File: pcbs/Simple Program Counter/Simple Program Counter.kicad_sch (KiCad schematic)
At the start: 0 parts

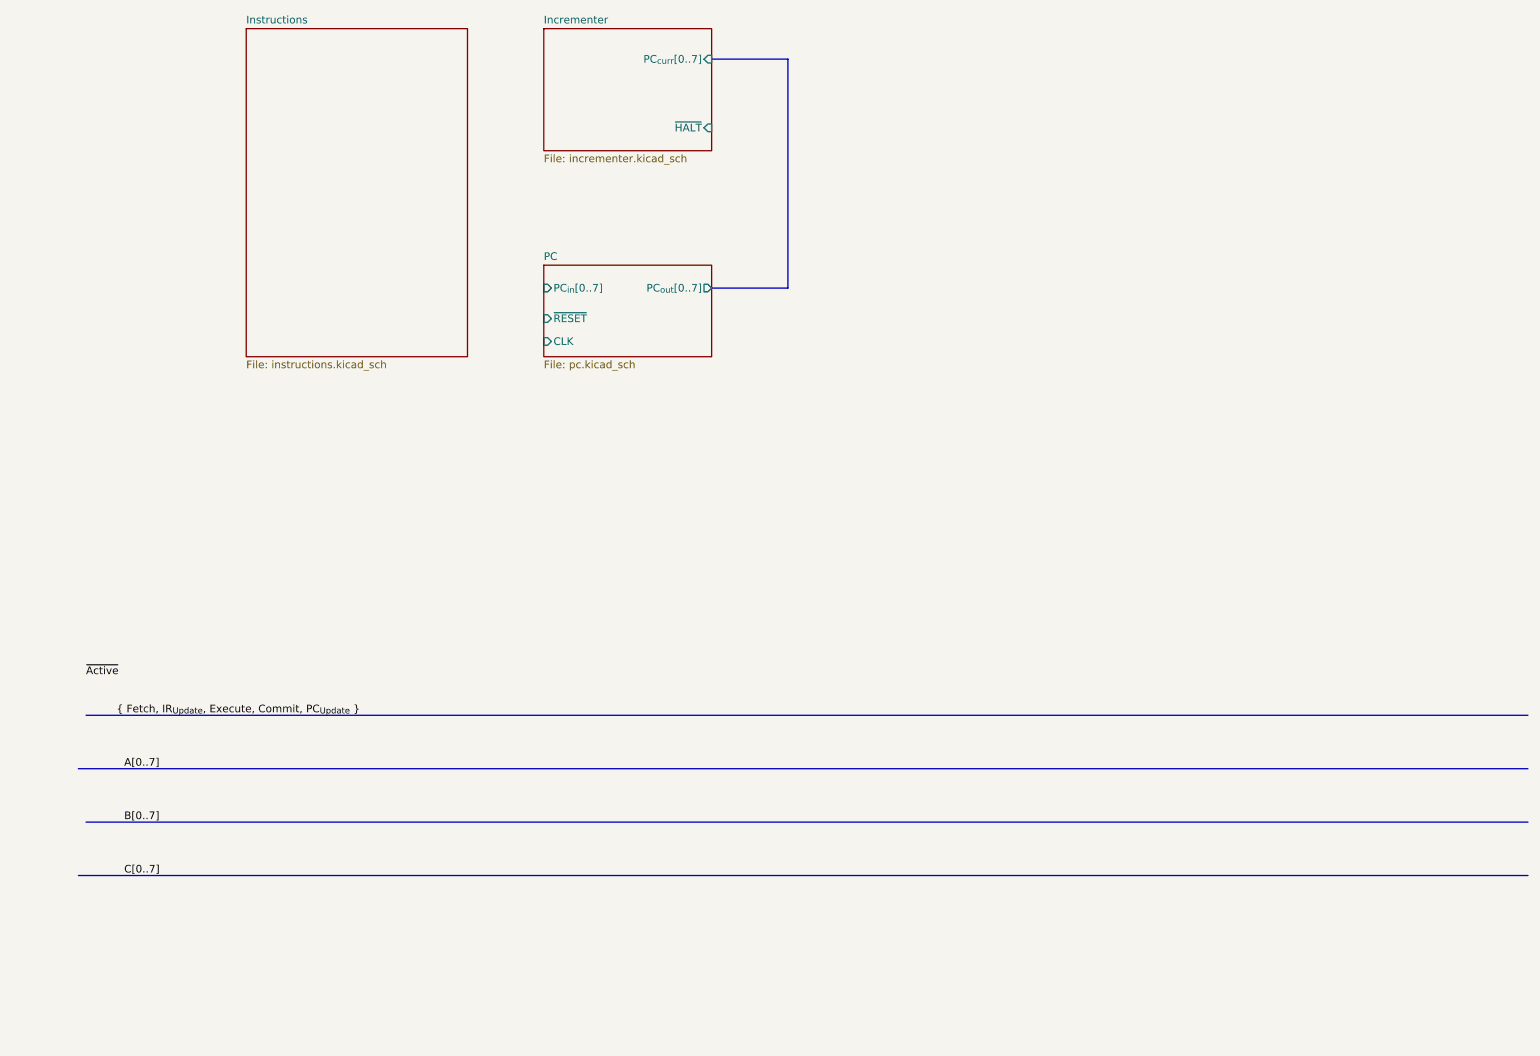
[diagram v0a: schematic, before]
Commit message: Getting close
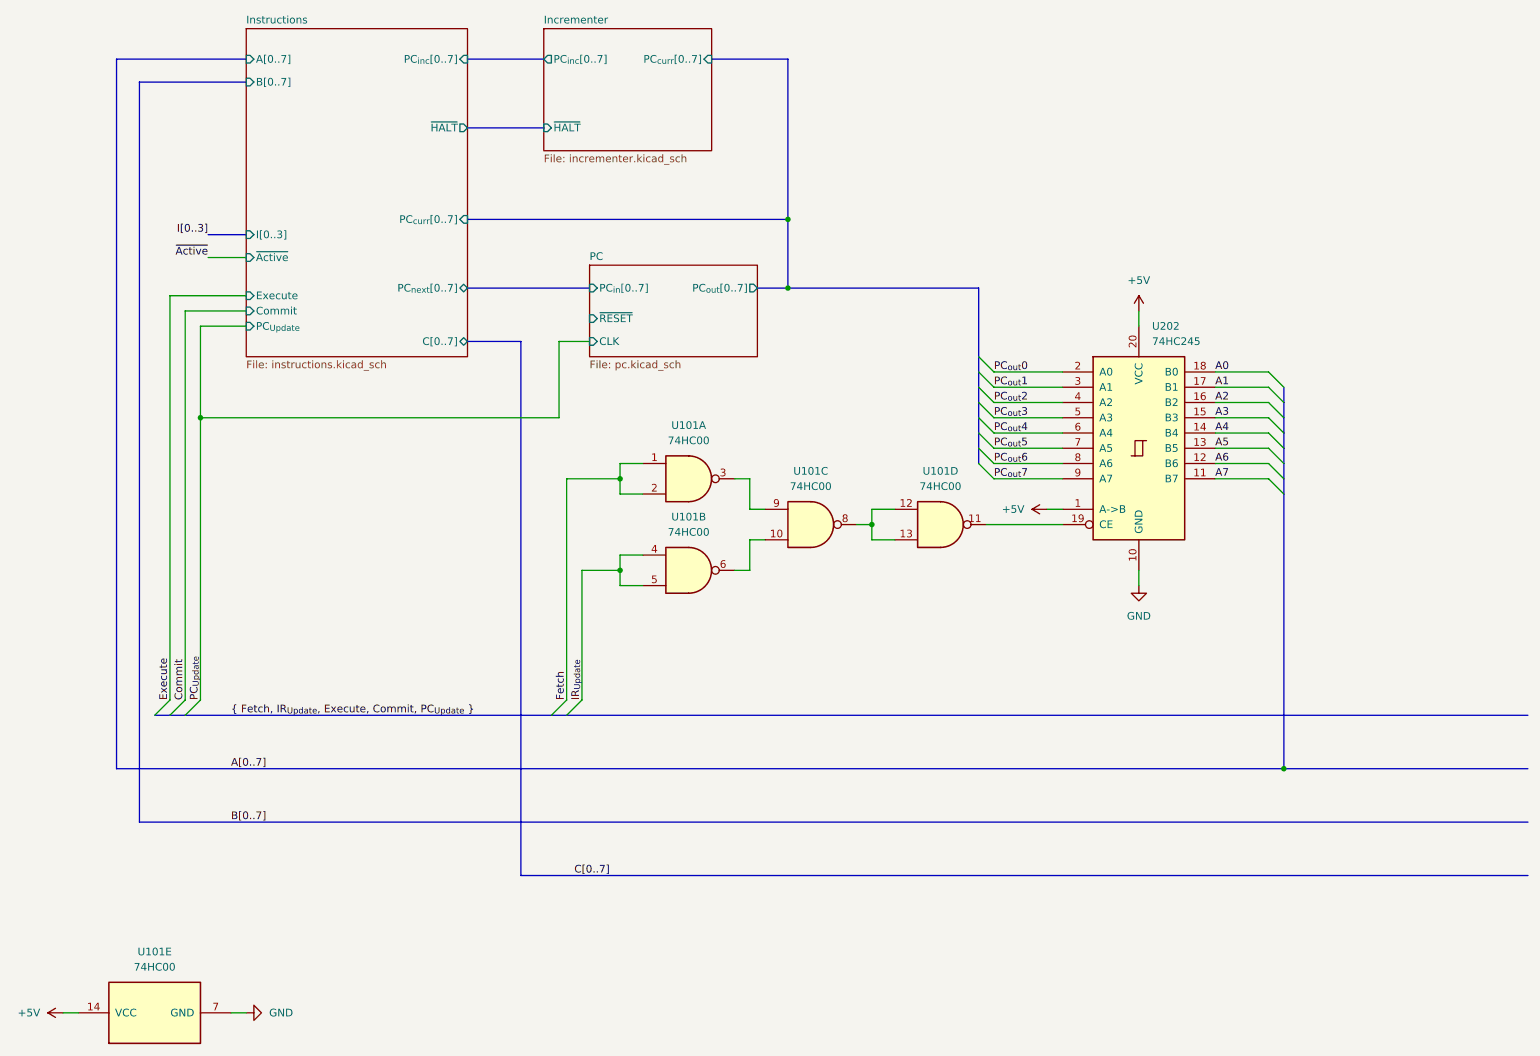
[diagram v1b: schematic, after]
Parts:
- added U101: 74HC00, Package_DIP:DIP-14_W7.62mm_Socket, symbol 74xx:74HC00
- added U202: 74HC245, Package_SO:SOIC-20W_7.5x12.8mm_P1.27mm, symbol 74xx:74HC245
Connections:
- new net: U101.10, U101.6
- new net: U101.3, U101.9
- new net: U101.12, U101.13, U101.8
- new net: U101.11, U202.19 (CE)
- new net +5V: U101.14 (VCC), U202.1 (A->B), U202.20 (VCC)
- new net A0: U202.18 (B0)
- new net A1: U202.17 (B1)
- new net A2: U202.16 (B2)
- new net A3: U202.15 (B3)
- new net A4: U202.14 (B4)
- new net A5: U202.13 (B5)
- new net A6: U202.12 (B6)
- new net A7: U202.11 (B7)
- new net Fetch: U101.1, U101.2
- new net GND: U101.7 (GND), U202.10 (GND)
- new net IR_{Update}: U101.4, U101.5
- new net PC_{out}0: U202.2 (A0)
- new net PC_{out}1: U202.3 (A1)
- new net PC_{out}2: U202.4 (A2)
- new net PC_{out}3: U202.5 (A3)
- new net PC_{out}4: U202.6 (A4)
- new net PC_{out}5: U202.7 (A5)
- new net PC_{out}6: U202.8 (A6)
- new net PC_{out}7: U202.9 (A7)
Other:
- sheet Incrementer ports: added PC_{inc}[0..7]; removed none
- sheet Instructions ports: added A[0..7], B[0..7], C[0..7], Commit, Execute, I[0..3], PC_{Update}, PC_{curr}[0..7], PC_{inc}[0..7], PC_{next}[0..7], ~{Active}, ~{HALT}; removed none
